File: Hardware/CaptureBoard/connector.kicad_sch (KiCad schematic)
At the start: 1 part, among them J100 Conn_01x30_MountingPin

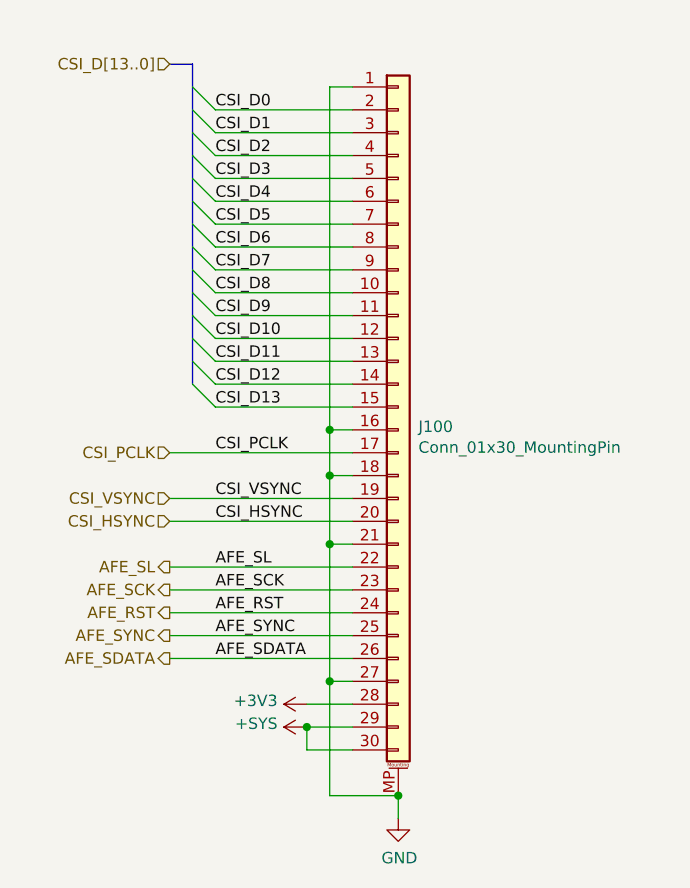
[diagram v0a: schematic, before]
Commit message: pcb: switch to ad9978 wip
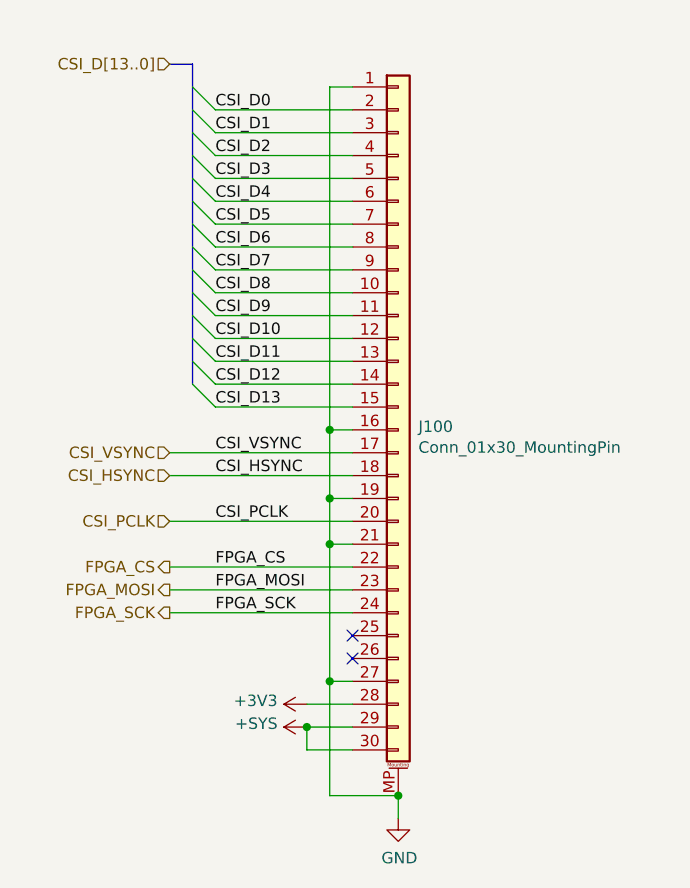
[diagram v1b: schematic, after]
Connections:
- net CSI_HSYNC: now also J100.18 (Pin_18); no longer J100.20 (Pin_20)
- net CSI_PCLK: now also J100.20 (Pin_20); no longer J100.17 (Pin_17)
- net CSI_VSYNC: now also J100.17 (Pin_17); no longer J100.19 (Pin_19)
- net GND: now also J100.19 (Pin_19); no longer J100.18 (Pin_18)
- net AFE_RST renamed FPGA_SCK
- net AFE_SCK renamed FPGA_MOSI
- net AFE_SDATA: no longer names the net of J100.26 (Pin_26)
- net AFE_SL renamed FPGA_CS
- net AFE_SYNC: no longer names the net of J100.25 (Pin_25)
- no-connect marks 0 -> 2
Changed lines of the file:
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@@
-(kicad_sch (version 20210126) (generator eeschema)
+(kicad_sch (version 20210621) (generator eeschema)
   (paper "A4")
   (junction (at 152.4 134.62) (diameter 0.9144) (color 0 0 0 0))
   (junction (at 154.94 101.6) (diameter 0.9144) (color 0 0 0 0))
-  (junction (at 154.94 106.68) (diameter 0.9144) (color 0 0 0 0))
+  (junction (at 154.94 109.22) (diameter 0.9144) (color 0 0 0 0))
   (junction (at 154.94 114.3) (diameter 0.9144) (color 0 0 0 0))
   (junction (at 154.94 129.54) (diameter 0.9144) (color 0 0 0 0))
   (junction (at 162.56 142.24) (diameter 0.9144) (color 0 0 0 0))
+  (no_connect (at 157.48 124.46))
+  (no_connect (at 157.48 127))
   (bus_entry (at 139.7 63.5) (size 2.54 2.54)
     (stroke (width 0.1524) (type solid) (color 0 0 0 0))
@@
     (stroke (width 0) (type solid) (color 0 0 0 0))
   )
-  (wire (pts (xy 137.16 109.22) (xy 157.48 109.22))
+  (wire (pts (xy 137.16 106.68) (xy 157.48 106.68))
     (stroke (width 0) (type solid) (color 0 0 0 0))
   )
@@
     (stroke (width 0) (type solid) (color 0 0 0 0))
   )
-  (wire (pts (xy 137.16 124.46) (xy 157.48 124.46))
-    (stroke (width 0) (type solid) (color 0 0 0 0))
-  )
-  (wire (pts (xy 137.16 127) (xy 157.48 127))
-    (stroke (width 0) (type solid) (color 0 0 0 0))
-  )
   (wire (pts (xy 142.24 66.04) (xy 157.48 66.04))
     (stroke (width 0) (type solid) (color 0 0 0 0))
@@
     (stroke (width 0) (type solid) (color 0 0 0 0))
   )
-  (wire (pts (xy 154.94 106.68) (xy 154.94 101.6))
-    (stroke (width 0) (type solid) (color 0 0 0 0))
-  )
-  (wire (pts (xy 154.94 114.3) (xy 154.94 106.68))
+  (wire (pts (xy 154.94 101.6) (xy 154.94 109.22))
+    (stroke (width 0) (type solid) (color 0 0 0 0))
+  )
+  (wire (pts (xy 154.94 114.3) (xy 154.94 109.22))
     (stroke (width 0) (type solid) (color 0 0 0 0))
   )
@@
     (stroke (width 0) (type solid) (color 0 0 0 0))
   )
-  (wire (pts (xy 157.48 106.68) (xy 154.94 106.68))
+  (wire (pts (xy 157.48 109.22) (xy 154.94 109.22))
     (stroke (width 0) (type solid) (color 0 0 0 0))
   )
@@
     (stroke (width 0) (type solid) (color 0 0 0 0))
   )
-  (bus (pts (xy 139.7 60.96) (xy 139.7 63.5))
-    (stroke (width 0) (type solid) (color 0 0 0 0))
-  )
-  (bus (pts (xy 139.7 63.5) (xy 139.7 66.04))
-    (stroke (width 0) (type solid) (color 0 0 0 0))
-  )
-  (bus (pts (xy 139.7 66.04) (xy 139.7 68.58))
-    (stroke (width 0) (type solid) (color 0 0 0 0))
-  )
-  (bus (pts (xy 139.7 68.58) (xy 139.7 71.12))
-    (stroke (width 0) (type solid) (color 0 0 0 0))
-  )
-  (bus (pts (xy 139.7 71.12) (xy 139.7 73.66))
-    (stroke (width 0) (type solid) (color 0 0 0 0))
-  )
-  (bus (pts (xy 139.7 73.66) (xy 139.7 76.2))
-    (stroke (width 0) (type solid) (color 0 0 0 0))
-  )
-  (bus (pts (xy 139.7 76.2) (xy 139.7 78.74))
-    (stroke (width 0) (type solid) (color 0 0 0 0))
-  )
-  (bus (pts (xy 139.7 78.74) (xy 139.7 81.28))
-    (stroke (width 0) (type solid) (color 0 0 0 0))
-  )
-  (bus (pts (xy 139.7 81.28) (xy 139.7 83.82))
-    (stroke (width 0) (type solid) (color 0 0 0 0))
-  )
-  (bus (pts (xy 139.7 83.82) (xy 139.7 86.36))
-    (stroke (width 0) (type solid) (color 0 0 0 0))
-  )
-  (bus (pts (xy 139.7 86.36) (xy 139.7 88.9))
-    (stroke (width 0) (type solid) (color 0 0 0 0))
-  )
-  (bus (pts (xy 139.7 88.9) (xy 139.7 91.44))
-    (stroke (width 0) (type solid) (color 0 0 0 0))
-  )
-  (bus (pts (xy 139.7 91.44) (xy 139.7 93.98))
-    (stroke (width 0) (type solid) (color 0 0 0 0))
-  )
-  (bus (pts (xy 139.7 93.98) (xy 139.7 96.52))
+  (bus (pts (xy 139.7 60.96) (xy 139.7 96.52))
     (stroke (width 0) (type solid) (color 0 0 0 0))
   )
@@
     (effects (font (size 1.27 1.27)) (justify left bottom))
   )
-  (label "CSI_PCLK" (at 142.24 104.14 0)
-    (effects (font (size 1.27 1.27)) (justify left bottom))
-  )
-  (label "CSI_VSYNC" (at 142.24 109.22 0)
-    (effects (font (size 1.27 1.27)) (justify left bottom))
-  )
-  (label "CSI_HSYNC" (at 142.24 111.76 0)
-    (effects (font (size 1.27 1.27)) (justify left bottom))
-  )
-  (label "AFE_SL" (at 142.24 116.84 0)
-    (effects (font (size 1.27 1.27)) (justify left bottom))
-  )
-  (label "AFE_SCK" (at 142.24 119.38 0)
-    (effects (font (size 1.27 1.27)) (justify left bottom))
-  )
-  (label "AFE_RST" (at 142.24 121.92 0)
-    (effects (font (size 1.27 1.27)) (justify left bottom))
-  )
-  (label "AFE_SYNC" (at 142.24 124.46 0)
-    (effects (font (size 1.27 1.27)) (justify left bottom))
-  )
-  (label "AFE_SDATA" (at 142.24 127 0)
+  (label "CSI_VSYNC" (at 142.24 104.14 0)
+    (effects (font (size 1.27 1.27)) (justify left bottom))
+  )
+  (label "CSI_HSYNC" (at 142.24 106.68 0)
+    (effects (font (size 1.27 1.27)) (justify left bottom))
+  )
+  (label "CSI_PCLK" (at 142.24 111.76 0)
+    (effects (font (size 1.27 1.27)) (justify left bottom))
+  )
+  (label "FPGA_CS" (at 142.24 116.84 0)
+    (effects (font (size 1.27 1.27)) (justify left bottom))
+  )
+  (label "FPGA_MOSI" (at 142.24 119.38 0)
+    (effects (font (size 1.27 1.27)) (justify left bottom))
+  )
+  (label "FPGA_SCK" (at 142.24 121.92 0)
     (effects (font (size 1.27 1.27)) (justify left bottom))
   )
@@
     (effects (font (size 1.27 1.27)) (justify right))
   )
-  (hierarchical_label "CSI_PCLK" (shape input) (at 137.16 104.14 180)
-    (effects (font (size 1.27 1.27)) (justify right))
-  )
-  (hierarchical_label "CSI_VSYNC" (shape input) (at 137.16 109.22 180)
-    (effects (font (size 1.27 1.27)) (justify right))
-  )
-  (hierarchical_label "CSI_HSYNC" (shape input) (at 137.16 111.76 180)
-    (effects (font (size 1.27 1.27)) (justify right))
-  )
-  (hierarchical_label "AFE_SL" (shape output) (at 137.16 116.84 180)
-    (effects (font (size 1.27 1.27)) (justify right))
-  )
-  (hierarchical_label "AFE_SCK" (shape output) (at 137.16 119.38 180)
-    (effects (font (size 1.27 1.27)) (justify right))
-  )
-  (hierarchical_label "AFE_RST" (shape output) (at 137.16 121.92 180)
-    (effects (font (size 1.27 1.27)) (justify right))
-  )
-  (hierarchical_label "AFE_SYNC" (shape output) (at 137.16 124.46 180)
-    (effects (font (size 1.27 1.27)) (justify right))
-  )
-  (hierarchical_label "AFE_SDATA" (shape output) (at 137.16 127 180)
-    (effects (font (size 1.27 1.27)) (justify right))
-  )
+  (hierarchical_label "CSI_VSYNC" (shape input) (at 137.16 104.14 180)
+    (effects (font (size 1.27 1.27)) (justify right))
+  )
+  (hierarchical_label "CSI_HSYNC" (shape input) (at 137.16 106.68 180)
+    (effects (font (size 1.27 1.27)) (justify right))
+  )
+  (hierarchical_label "CSI_PCLK" (shape input) (at 137.16 111.76 180)
+    (effects (font (size 1.27 1.27)) (justify right))
+  )
+  (hierarchical_label "FPGA_CS" (shape output) (at 137.16 116.84 180)
+    (effects (font (size 1.27 1.27)) (justify right))
+  )
+  (hierarchical_label "FPGA_MOSI" (shape output) (at 137.16 119.38 180)
+    (effects (font (size 1.27 1.27)) (justify right))
+  )
+  (hierarchical_label "FPGA_SCK" (shape output) (at 137.16 121.92 180)
+    (effects (font (size 1.27 1.27)) (justify right))
+  )

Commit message: pcb: PB r0p2 and CB r0p3 freeze
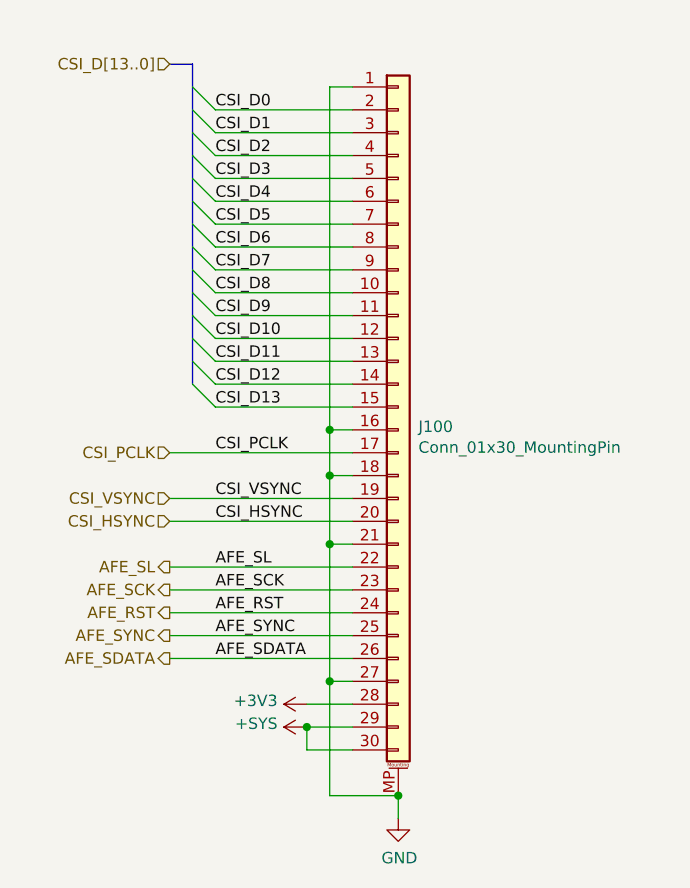
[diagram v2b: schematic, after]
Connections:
- net CSI_HSYNC: now also J100.20 (Pin_20); no longer J100.18 (Pin_18)
- net CSI_PCLK: now also J100.17 (Pin_17); no longer J100.20 (Pin_20)
- net CSI_VSYNC: now also J100.19 (Pin_19); no longer J100.17 (Pin_17)
- net GND: now also J100.18 (Pin_18); no longer J100.19 (Pin_19)
- net AFE_SYNC: now reaches J100.25 (Pin_25)
- net AFE_SDATA: now reaches J100.26 (Pin_26)
- net FPGA_CS renamed AFE_SL
- net FPGA_MOSI renamed AFE_SCK
- net FPGA_SCK renamed AFE_RST
- no-connect marks 2 -> 0

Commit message: pcb: CB r0p4
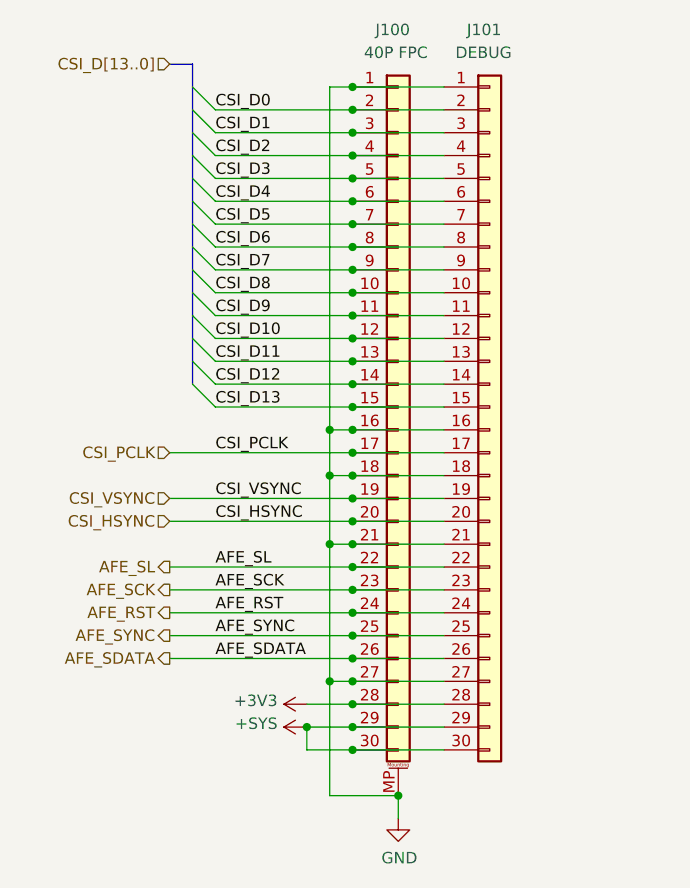
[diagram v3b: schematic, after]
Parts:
- added J101: DEBUG, Connector_PinHeader_2.00mm:PinHeader_2x15_P2.00mm_Vertical, symbol Connector_Generic:Conn_01x30
- J100: value Conn_01x30_MountingPin -> 40P FPC
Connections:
- net +3V3: now also J101.28 (Pin_28)
- net +SYS: now also J101.29 (Pin_29), J101.30 (Pin_30)
- net AFE_RST: now also J101.24 (Pin_24)
- net AFE_SCK: now also J101.23 (Pin_23)
- net AFE_SDATA: now also J101.26 (Pin_26)
- net AFE_SL: now also J101.22 (Pin_22)
- net AFE_SYNC: now also J101.25 (Pin_25)
- net CSI_D0: now also J101.2 (Pin_2)
- net CSI_D1: now also J101.3 (Pin_3)
- net CSI_D10: now also J101.12 (Pin_12)
- net CSI_D11: now also J101.13 (Pin_13)
- net CSI_D12: now also J101.14 (Pin_14)
- net CSI_D13: now also J101.15 (Pin_15)
- net CSI_D2: now also J101.4 (Pin_4)
- net CSI_D3: now also J101.5 (Pin_5)
- net CSI_D4: now also J101.6 (Pin_6)
- net CSI_D5: now also J101.7 (Pin_7)
- net CSI_D6: now also J101.8 (Pin_8)
- net CSI_D7: now also J101.9 (Pin_9)
- net CSI_D8: now also J101.10 (Pin_10)
- net CSI_D9: now also J101.11 (Pin_11)
- net CSI_HSYNC: now also J101.20 (Pin_20)
- net CSI_PCLK: now also J101.17 (Pin_17)
- net CSI_VSYNC: now also J101.19 (Pin_19)
- net GND: now also J101.1 (Pin_1), J101.16 (Pin_16), J101.18 (Pin_18), J101.21 (Pin_21), J101.27 (Pin_27)
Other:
- title: (none) -> SitinaNe
